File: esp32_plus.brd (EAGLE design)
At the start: 86.4 x 76.2 mm, 27 parts, among them U1 ESP32 DEVKIT-V4

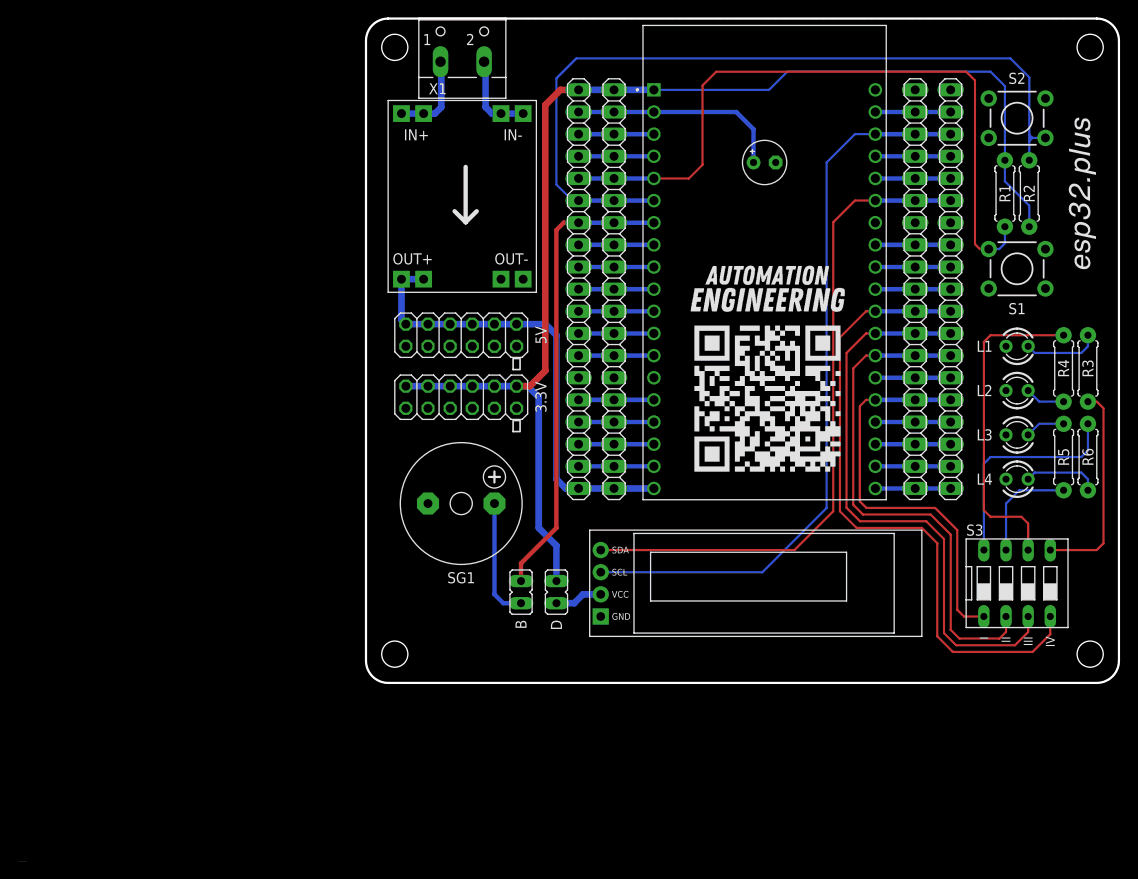
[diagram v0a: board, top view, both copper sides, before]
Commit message: Add files via upload
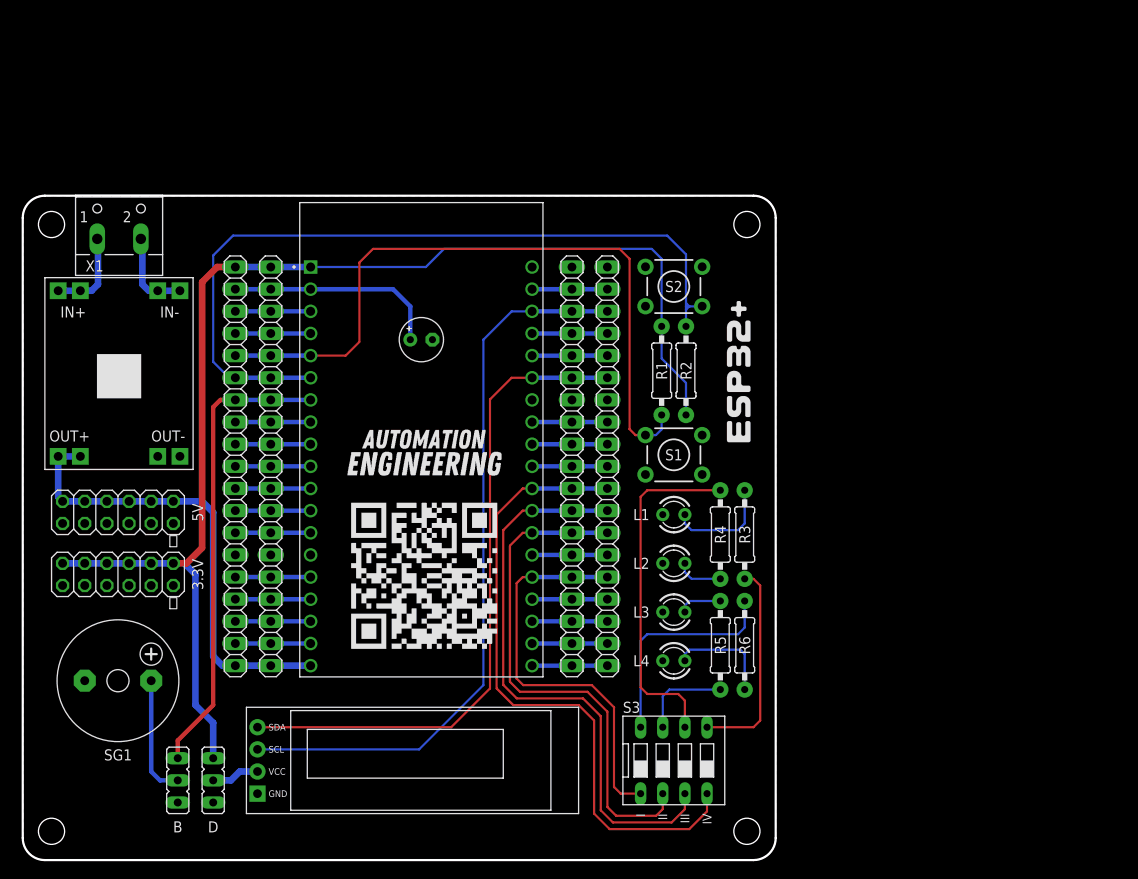
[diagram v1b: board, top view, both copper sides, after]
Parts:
- B, D: device jumper:JP1 -> jumper_edit:JP2
- R1, R2, R3, R4, R5, R6: device rcl_Edit:0207/7 -> rcl_Edit:0207/10
- moved R6 44.9 mm to (82.8, 24.6)
- moved B 44.9 mm to (17.8, 9.14), turned to 270 degrees
- moved D 44.9 mm to (21.8, 9.14), turned to 90 degrees
- moved R5 44.9 mm to (80.0, 24.6)
- moved S1 44.8 mm to (74.7, 46.5)
- moved L4 44.5 mm to (74.7, 22.9)
- moved C1 44.3 mm to (45.7, 59.7)
- moved 3.3V 44.3 mm to (10.9, 32.8)
- moved 5V 44.3 mm to (10.9, 39.9)
- moved L3 44.3 mm to (74.7, 28.4)
- moved MA_JP3 44.3 mm to (67.1, 45.2)
- moved R1 44.3 mm to (73.3, 56.1)
- moved R2 44.3 mm to (76.1, 56.1)
- moved S3 44.3 mm to (74.7, 11.4)
- moved SG1 44.3 mm to (10.9, 20.6)
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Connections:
- net 3V3: now also D.3; no longer D.2
- net N$1: now also D.2; no longer D.1
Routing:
- net N$17: track 8.76 -> 12.3 mm
- net N$20: track 8.76 -> 12.1 mm
- net N$2: track 37.5 -> 40.1 mm
- net N$3: track 12.6 -> 10.5 mm
- net 3V3: track 144.5 -> 146.0 mm
- net GPIO35_X: track 92.6 -> 91.4 mm
- net N$18: track 4.59 -> 5.40 mm
- net GPIO34_X: track 80.9 -> 81.5 mm
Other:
- board text removed: "D:/Download/esp32_plus.bmp"
- board text removed: "D:/Download/moe.bmp"
